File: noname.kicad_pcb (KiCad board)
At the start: 2 copper layers, 140.3 x 107.2 mm, 103 parts, among them J1 TRRS, J2 battery, SW0 SW_PUSH, SW1 SW_PUSH, SW10 SW_PUSH, SW11 SW_PUSH, SW12 SW_PUSH, SW13 SW_PUSH, SW14 SW_PUSH, SW15 SW_PUSH, SW16 SW_PUSH, SW17 SW_PUSH, SW18 SW_PUSH, SW19 SW_PUSH, SW2 SW_PUSH, SW20 SW_PUSH, SW21 SW_PUSH, SW22 SW_PUSH, SW23 SW_PUSH, SW24 SW_PUSH, SW25 SW_PUSH, SW26 SW_PUSH, SW27 SW_PUSH, SW28 SW_PUSH, SW29 SW_PUSH, SW3 SW_PUSH, SW30 SW_PUSH, SW4 SW_PUSH, SW5 SW_PUSH, SW6 SW_PUSH, SW7 SW_PUSH, SW8 SW_PUSH, SW9 SW_PUSH, SW91 SW_SPDT, U0 ProMicro, U1 HOLE, U2 HOLE, U3 HOLE, U4 HOLE, U5 HOLE

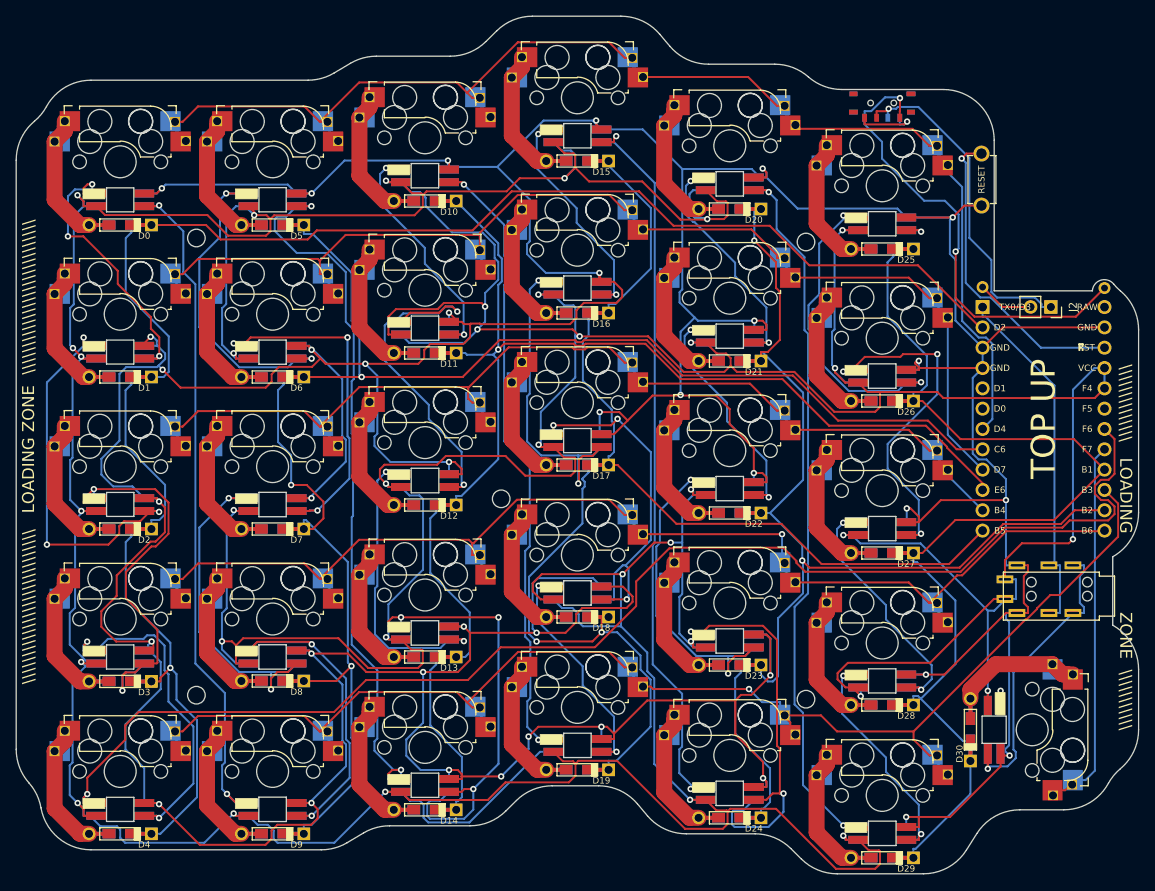
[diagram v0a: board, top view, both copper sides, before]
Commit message: missing silk
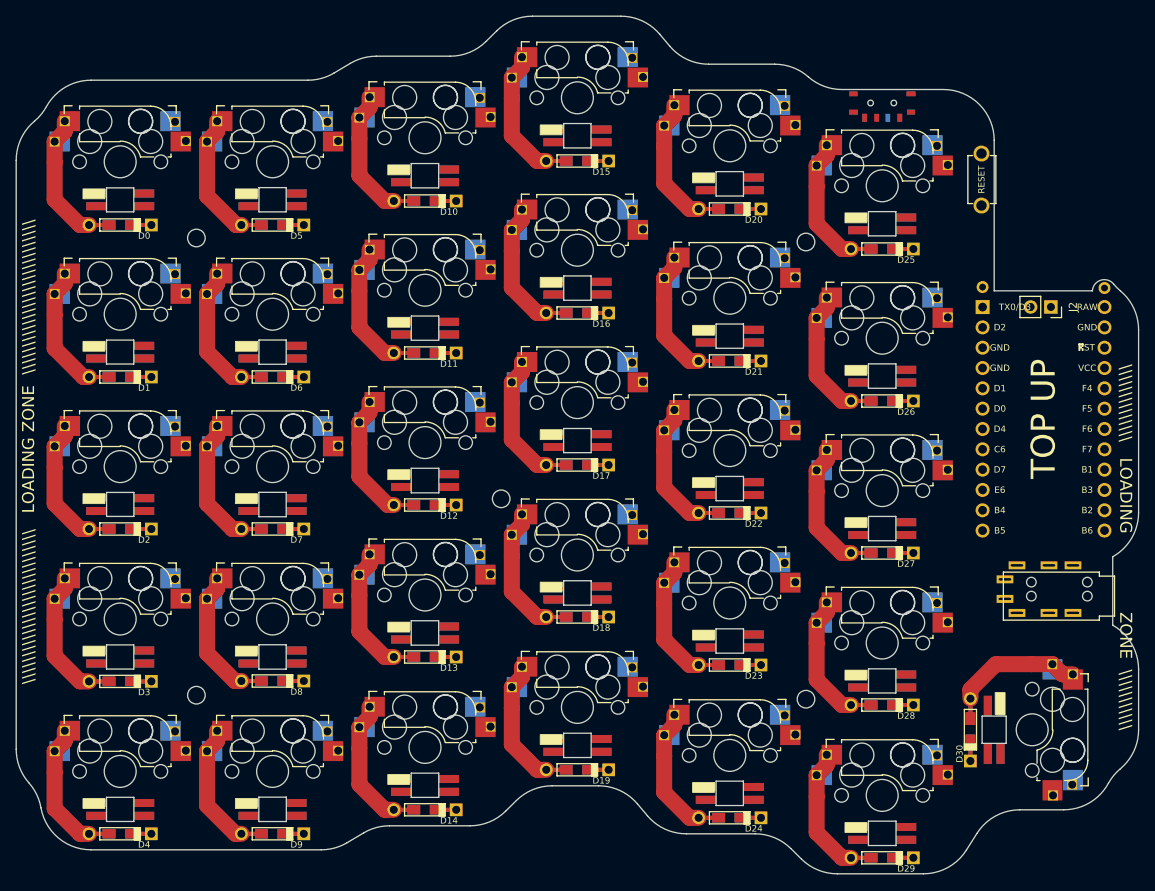
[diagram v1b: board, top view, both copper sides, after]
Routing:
- net VCC: track 978.0 -> 0.00 mm, vias 35 -> 0
- net GND: track 872.4 -> 0.00 mm, vias 38 -> 0
- net COL0: track 233.6 -> 0.00 mm, vias 1 -> 0
- net COL1: track 217.7 -> 0.00 mm, vias 3 -> 0
- net COL2: track 188.1 -> 0.00 mm, vias 1 -> 0
- net COL3: track 184.0 -> 0.00 mm, vias 2 -> 0
- net ROW4: track 178.9 -> 0.00 mm, vias 1 -> 0
- net ROW0: track 170.1 -> 0.00 mm
- net LED: track 169.6 -> 0.00 mm, vias 1 -> 0
- net COL4: track 163.5 -> 0.00 mm, vias 2 -> 0
- net ROW3: track 161.0 -> 0.00 mm, vias 1 -> 0
- net COL5: track 156.6 -> 0.00 mm
- net ROW1: track 154.3 -> 0.00 mm
- net ROW2: track 141.2 -> 0.00 mm
- net Net-(D915-Pad1): track 94.1 -> 0.00 mm, vias 2 -> 0
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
